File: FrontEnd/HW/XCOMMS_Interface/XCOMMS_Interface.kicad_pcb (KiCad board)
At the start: 4 copper layers, 40 x 65 mm, 100 parts, among them J1 TFC-110-02-F-D-A-P-FR, J2 UART, J3 JTAG, J4 12V, U1 STM32L431KBUx, U10 MAX870EUK, U2 TPS56637, U3 TPS56637, U4 TPS56637, U5 TPS784, U6 MAX870EUK, U7 INA290, U8 AD5160, U9 MAX870EUK, Y1 TCXO_ECS

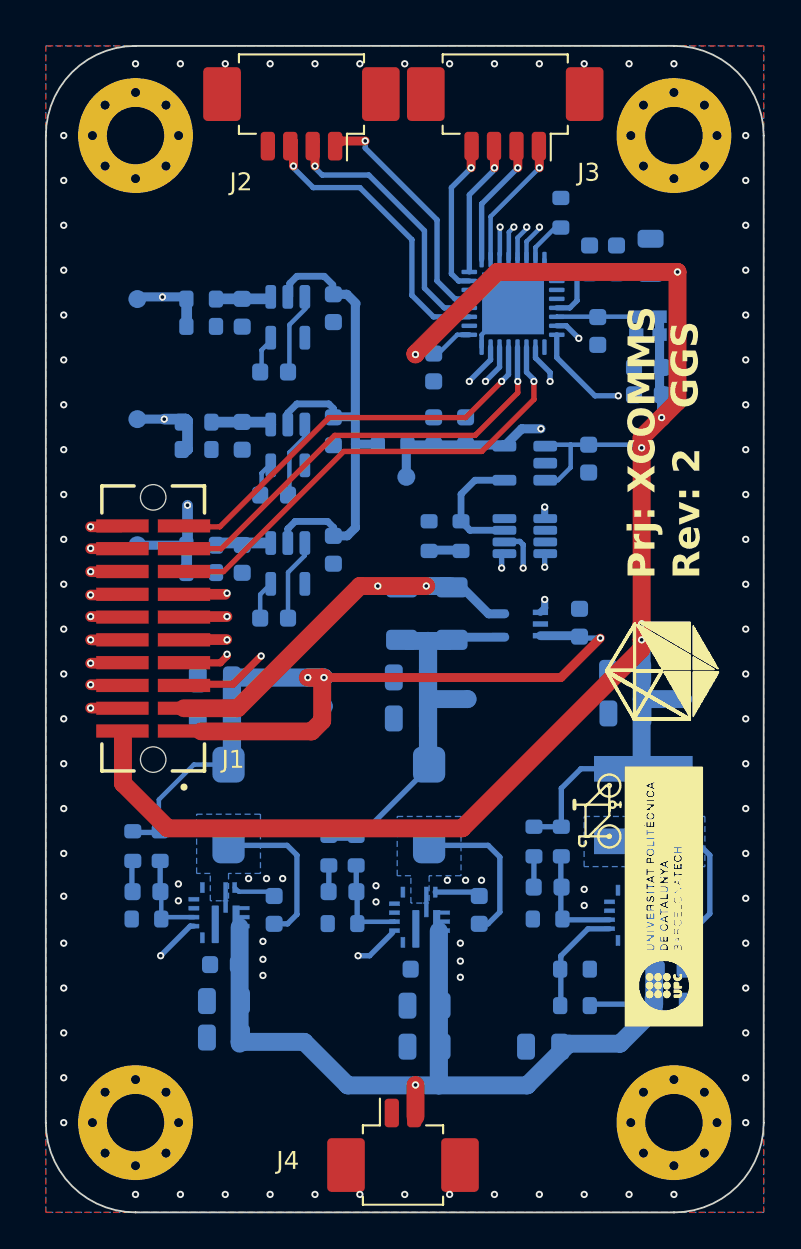
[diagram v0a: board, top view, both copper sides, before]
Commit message: XCOMMS RF update and PA EvalBoard
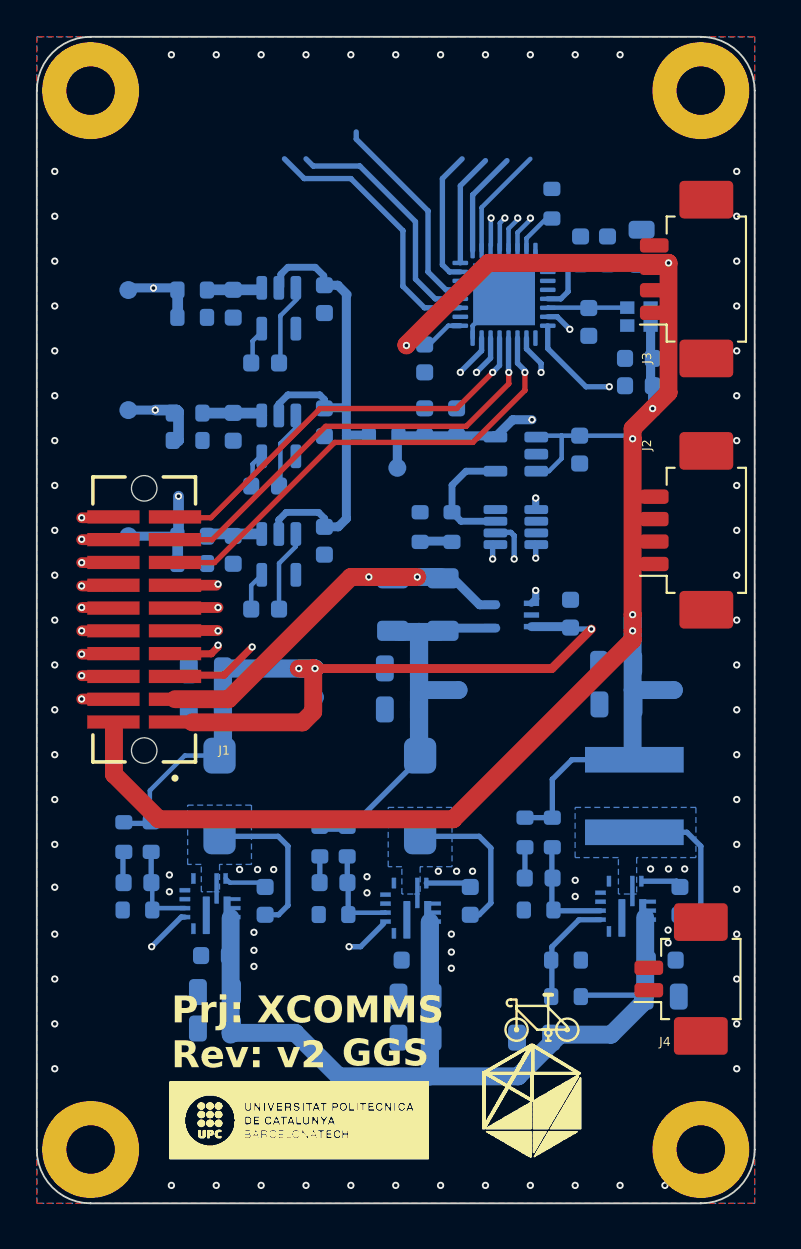
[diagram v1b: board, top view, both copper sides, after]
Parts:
- SCRW1, SCRW2, SCRW3, SCRW4: footprint MountingHole:MountingHole_3.2mm_M3_Pad_Via -> MountingHole:MountingHole_2.7mm_M2.5_Pad
- moved Designator7 40.3 mm to (135.6, 129.6), turned to 0 degrees
- moved Designator6 36.8 mm to (135.5, 127.1), turned to 0 degrees
- moved J2 32.5 mm to (164.8, 99.5), turned to 90 degrees
- moved Designator9 30.6 mm to (135.4, 134.5), turned to 0 degrees
- moved Designator8 28.9 mm to (142.9, 135.6), turned to 0 degrees
- moved J4 18.9 mm to (164.5, 124.5), turned to 90 degrees
- moved J3 14.5 mm to (164.8, 85.5), turned to 90 degrees
- moved SCRW3 3.54 mm to (131.0, 75.0)
- moved SCRW4 2.92 mm to (165.0, 75.0)
- moved SCRW1 2.91 mm to (131.0, 134.0)
- moved SCRW2 2.12 mm to (165.0, 134.0)
- moved C1 0.71 mm to (161.7, 83.7)
- moved C10 0.71 mm to (137.9, 127.3)
- moved C11 0.71 mm to (137.9, 125.2)
- moved C13 0.71 mm to (155.7, 127.8)
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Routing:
- net +12V: track 50.9 -> 49.1 mm, vias 1 -> 0
- net /USART1_CTS: track 13.3 -> 11.7 mm, vias 1 -> 0
- net /JTDI: track 7.34 -> 5.81 mm, vias 1 -> 0
- net /JTDO: track 7.75 -> 6.24 mm, vias 1 -> 0
- net /JTCK: track 7.79 -> 6.28 mm, vias 1 -> 0
- net /JTMS: track 9.03 -> 7.52 mm, vias 1 -> 0
- net /USART1_Tx: track 16.5 -> 15.1 mm, vias 1 -> 0
- net /USART1_Rx: track 15.1 -> 13.7 mm, vias 1 -> 0
- net GND: vias 101 -> 94
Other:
- outline, holes or cut-outs redrawn
